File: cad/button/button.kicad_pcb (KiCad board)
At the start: 2 copper layers, 60 x 20 mm, 17 parts, among them J1 uSD_SPI, J2 SWD, SW1 SW_Push, U1 STM32L072KZTx, U2 PAM8302AAS

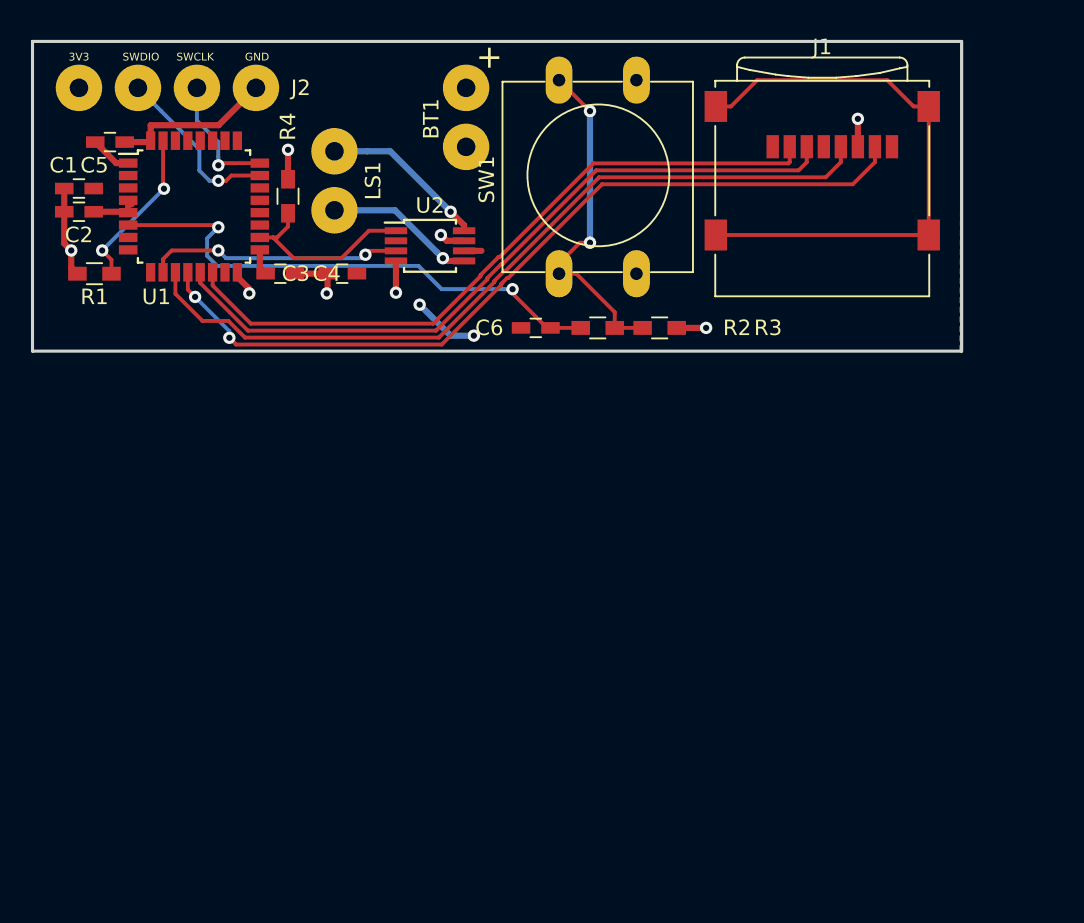
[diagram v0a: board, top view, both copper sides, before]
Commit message: more drawing
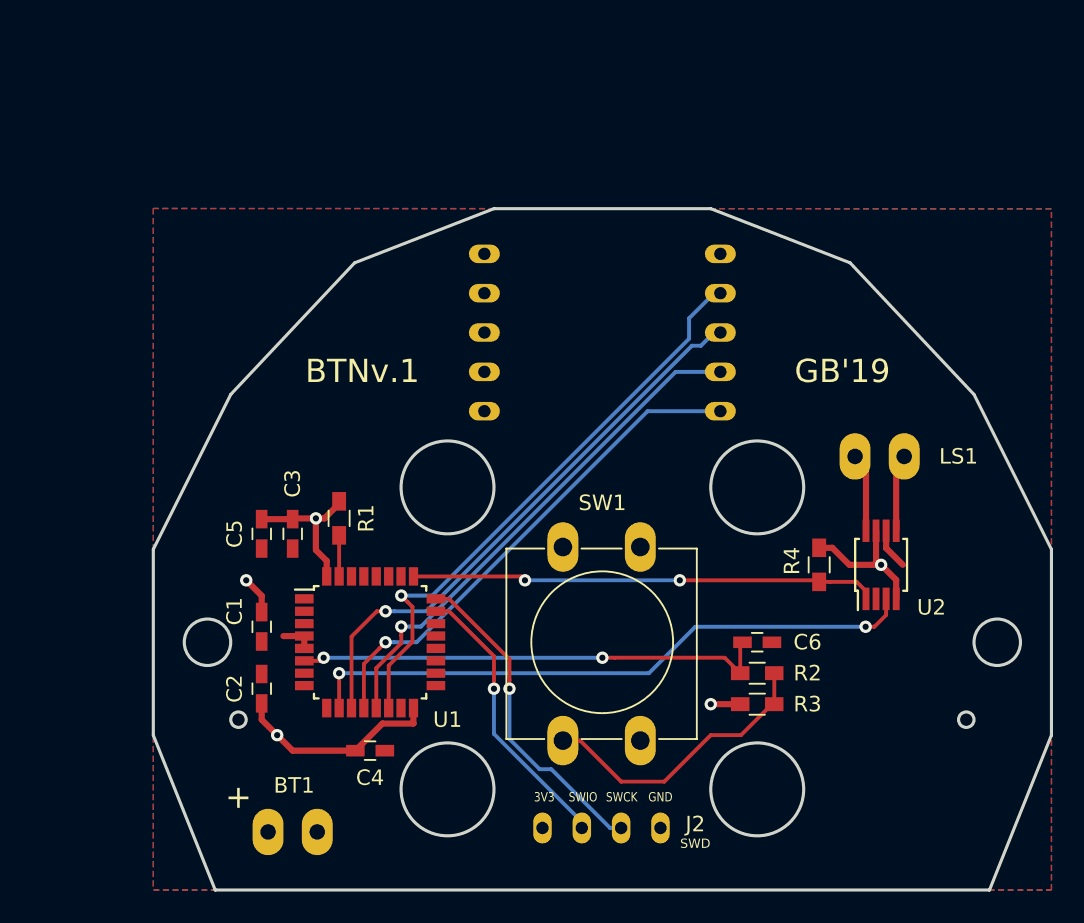
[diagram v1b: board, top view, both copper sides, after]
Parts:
- J1: footprint Connectors:microSD_Card_Receptacle_Wuerth_693072010801 -> custom:PJRC_uSD_Adapter; moved to B.Cu
- SW1: footprint Buttons_Switches_THT:SW_PUSH-12mm -> custom:SW_PUSH-12mm
- moved J2 57.4 mm to (52.8, 63.0), turned to 270 degrees
- moved BT1 47.5 mm to (29.0, 63.2), turned to 0 degrees
- moved R4 41.7 mm to (63.0, 46.0)
- moved LS1 39.4 mm to (66.9, 39.0), turned to 180 degrees
- moved U2 35.7 mm to (67.0, 46.0), turned to 90 degrees
- moved C2 33.0 mm to (27.0, 54.0), turned to 270 degrees
- moved C4 31.3 mm to (34.0, 58.0), turned to 0 degrees
- moved C1 30.7 mm to (27.0, 50.0), turned to 270 degrees
- moved U1 30.4 mm to (34.0, 51.0)
- moved SW1 30.2 mm to (46.5, 57.4)
- moved C5 27.1 mm to (27.0, 44.0), turned to 270 degrees
- moved R3 25.1 mm to (59.0, 55.0), turned to 180 degrees
- moved C6 24.8 mm to (59.0, 51.0), turned to 0 degrees
- moved R2 24.6 mm to (59.0, 53.0)
- moved R1 22.3 mm to (32.0, 43.0), turned to 90 degrees
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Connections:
- J1 pad 1: (no net) -> GND
- J1 pad 3: SD_MOSI -> SD_SCK
- J1 pad 4: +3V3 -> SD_MOSI
- J1 pad 5: SD_SCK -> SD_MISO
- J1 pad 6: GND -> (no net)
- J1 pad 7: SD_MISO -> (no net)
- J1 pad 9: Net-(J1-Pad9) -> (no net)
- U1 pad 18: SPK_SD -> Net-(U1-Pad18)
- U1 pad 25: Net-(U1-Pad25) -> SPK_SD
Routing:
- net Net-(J1-Pad9): track 37.2 -> 0.00 mm
- net SPK_IN: track 16.5 -> 40.2 mm
- net SD_MISO: track 53.1 -> 32.6 mm, vias 2 -> 1
- net SPK_SD: track 12.2 -> 30.1 mm, vias 0 -> 2
- net SD_SCK: track 51.3 -> 36.6 mm, vias 0 -> 1
- net SD_MOSI: track 46.7 -> 33.4 mm, vias 0 -> 1
- net /SWCLK: track 8.31 -> 21.1 mm
- net +3V3: track 14.3 -> 4.80 mm, vias 2 -> 0
- net /BOOT0: track 10.5 -> 2.65 mm, vias 2 -> 0
- net /SWDIO: track 11.4 -> 18.4 mm
- net SD_CS: track 44.5 -> 37.7 mm, vias 0 -> 1
- net /SPK_1: track 11.8 -> 5.01 mm, vias 1 -> 0
- net GND: track 30.8 -> 37.0 mm, vias 8 -> 5
- net /SPK_2: track 10.7 -> 5.09 mm, vias 1 -> 0
- net /SW_IN: track 34.2 -> 30.7 mm
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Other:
- board size 60 x 20 mm -> 58 x 44 mm
- board text added: "SWCK"
- board text added: "SWD"
- board text added: "SWIO"
- board text removed: "SWCLK"
- board text removed: "SWDIO"

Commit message: finish up schematic
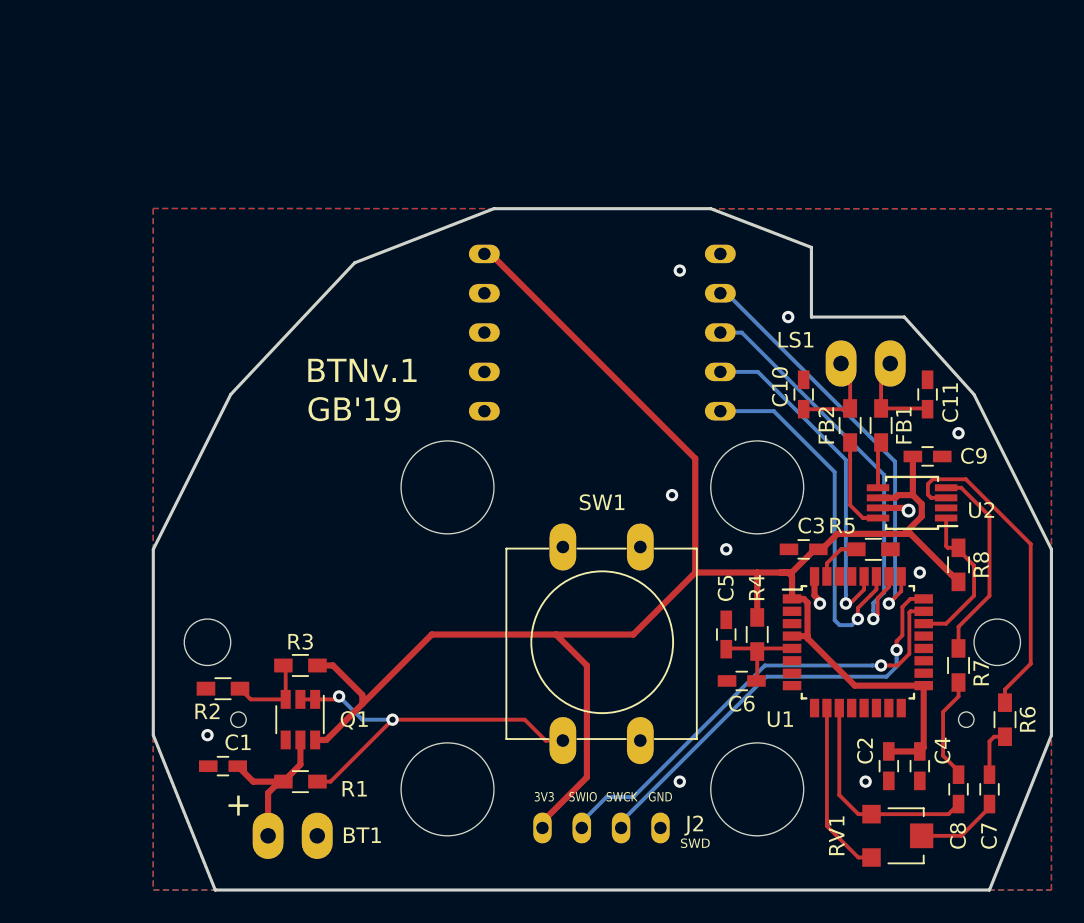
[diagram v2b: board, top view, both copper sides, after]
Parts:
- added C10: 220pF, Capacitors_SMD:C_0603_HandSoldering, F.Cu at (62.0, 35.0)
- added C11: 220pF, Capacitors_SMD:C_0603_HandSoldering, F.Cu at (70.0, 35.0)
- added C7: 1uF, Capacitors_SMD:C_0603_HandSoldering, F.Cu at (74.0, 60.5)
- added C8: 1uF, Capacitors_SMD:C_0603_HandSoldering, F.Cu at (72.0, 60.5)
- added C9: 10uF, Capacitors_SMD:C_0603_HandSoldering, F.Cu at (70.0, 39.0)
- added FB1: Ferrite_Bead_Small, Resistors_SMD:R_0603_HandSoldering, F.Cu at (67.0, 37.0)
- added FB2: Ferrite_Bead_Small, Resistors_SMD:R_0603_HandSoldering, F.Cu at (65.0, 37.0)
- added Q1: DMC2038LVT, TO_SOT_Packages_SMD:TSOT-23-6, F.Cu at (29.5, 56.0)
- added R5: 10K, Resistors_SMD:R_0603_HandSoldering, F.Cu at (66.5, 45.0)
- added R6: 10K, Resistors_SMD:R_0603_HandSoldering, F.Cu at (75.0, 56.0)
- added R7: 10K, Resistors_SMD:R_0603_HandSoldering, F.Cu at (72.0, 52.5)
- added R8: 10K, Resistors_SMD:R_0603_HandSoldering, F.Cu at (72.0, 46.0)
- added REF**: MountingHole_0.5mm, custom:MountingHole_0.5mm, F.Cu at (72.5, 56.0)
- added REF**: MountingHole_1.5mm, custom:MountingHole_1.5mm, F.Cu at (74.5, 51.0)
- added REF**: MountingHole_3mm, Mounting_Holes:MountingHole_3mm, F.Cu at (59.0, 60.5)
- added REF**: MountingHole_3mm, Mounting_Holes:MountingHole_3mm, F.Cu at (39.0, 60.5)
- added REF**: MountingHole_3mm, Mounting_Holes:MountingHole_3mm, F.Cu at (59.0, 41.0)
- added REF**: MountingHole_3mm, Mounting_Holes:MountingHole_3mm, F.Cu at (39.0, 41.0)
- added REF**: MountingHole_1.5mm, custom:MountingHole_1.5mm, F.Cu at (23.5, 51.0)
- added REF**: MountingHole_0.5mm, custom:MountingHole_0.5mm, F.Cu at (25.5, 56.0)
- added RV1: R_POT, Potentiometers:Potentiometer_Trimmer-EVM3E, F.Cu at (68.0, 63.5)
- C1: value 100nF -> 10uF
- C2: value 1uF -> 10uF
- C3: value 10uF -> 100nF
- C5: value 100nF -> 1uF
- R2: value 1K -> 10K
- R3: value 10K -> not fitted
- R4: value 10K -> 10
- SW1: value SW_Push -> Button; footprint custom:SW_PUSH-12mm -> Buttons_Switches_THT:SW_PUSH-12mm
- moved C2 40.8 mm to (67.5, 59.0)
- moved C4 35.5 mm to (69.5, 59.0), turned to 90 degrees
- moved R2 34.5 mm to (24.5, 54.0)
- moved C3 33.0 mm to (62.0, 45.0), turned to 0 degrees
- moved U1 31.5 mm to (65.5, 51.0)
- moved C5 30.7 mm to (57.0, 50.5)
- moved R3 29.6 mm to (29.5, 52.5)
- moved R1 17.2 mm to (29.5, 60.0), turned to 180 degrees
- moved C1 9.34 mm to (24.5, 59.0), turned to 180 degrees
- moved LS1 6.07 mm to (66.0, 33.0)
- moved R4 6.02 mm to (59.0, 50.5)
- moved U2 4.47 mm to (69.0, 42.0), turned to 180 degrees
- moved C6 2.69 mm to (58.0, 53.5)
- moved BT1 0.25 mm to (29.0, 63.5)
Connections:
- BT1 pad 1: +3V3 -> /VBAT
- C1 pad 1: GND -> /VBAT
- C1 pad 2: +3V3 -> GND
- C3 pad 1: +3V3 -> GND
- C3 pad 2: GND -> +3V3
- C5 pad 2: +3V3 -> /VDDA
- C6 pad 1: /SW_IN -> GND
- C6 pad 2: +3V3 -> /VDDA
- LS1 pad 1: /SPK_1 -> /SPK+
- LS1 pad 2: /SPK_2 -> /SPK-
- R1 pad 1: /BOOT0 -> /GATE_N
- R1 pad 2: GND -> /VBAT
- R2 pad 1: Net-(R2-Pad1) -> /GATE_P
- R2 pad 2: /SW_IN -> GND
- R3 pad 1: Net-(R2-Pad1) -> +3V3
- R3 pad 2: GND -> /GATE_P
- R4 pad 1: GND -> +3V3
- R4 pad 2: SPK_SD -> /VDDA
- SW1 pad 1: Net-(R2-Pad1) -> /GATE_N
- SW1 pad 2: +3V3 -> GND
- U1 pad 10: SPK_IN -> SPK_IN+
- U1 pad 11: SD_SCK -> SPK_IN-
- U1 pad 12: SD_MISO -> Net-(U1-Pad12)
- U1 pad 13: SD_MOSI -> Net-(U1-Pad13)
- U1 pad 14: SD_CS -> Net-(U1-Pad14)
- U1 pad 22: Net-(U1-Pad22) -> SPK_SD
- U1 pad 25: SPK_SD -> SD_CS
- U1 pad 26: Net-(U1-Pad26) -> SD_SCK
- U1 pad 27: Net-(U1-Pad27) -> SD_MISO
- U1 pad 28: Net-(U1-Pad28) -> SD_MOSI
- U1 pad 5: +3V3 -> /VDDA
- U1 pad 6: /SW_IN -> Net-(U1-Pad6)
- U2 pad 3: SPK_IN -> Net-(R6-Pad1)
- U2 pad 4: GND -> Net-(R7-Pad1)
- U2 pad 5: /SPK_1 -> Net-(FB1-Pad1)
- U2 pad 8: /SPK_2 -> Net-(FB2-Pad1)
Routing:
- net +3V3: track 4.80 -> 126.3 mm
- net SPK_IN: track 40.2 -> 0.00 mm, vias 2 -> 0
- net GND: track 37.0 -> 3.95 mm, vias 5 -> 11
- net /SW_IN: track 30.7 -> 0.00 mm, vias 2 -> 0
- net /GATE_N: track 0.00 -> 24.7 mm, vias 0 -> 2
- net Net-(R6-Pad1): track 0.00 -> 21.4 mm
- net SPK_SD: track 30.1 -> 10.2 mm, vias 2 -> 0
- net Net-(R2-Pad1): track 18.8 -> 0.00 mm
- net SPK_IN-: track 0.00 -> 14.1 mm
- net Net-(R7-Pad1): track 0.00 -> 12.9 mm
- net SPK_IN+: track 0.00 -> 11.3 mm
- net /SWDIO: track 18.4 -> 29.7 mm
- net SD_MOSI: track 33.4 -> 22.1 mm
- net /VBAT: track 0.00 -> 10.6 mm
- net SD_CS: track 37.7 -> 27.2 mm
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- added copper zone on F.Cu, net GND
- removed copper zone on F.Cu, net +3V3
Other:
- outline, holes or cut-outs redrawn
- net class 3V3 removed
- net class Power added: clearance 0.2, trace_width 0.4, via_dia 0.9, via_drill 0.5
